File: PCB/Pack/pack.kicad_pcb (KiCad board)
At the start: 2 copper layers, 100 x 100 mm, 45 parts, among them J1 Conn_01x01, J2 Conn_01x01, J3 Conn_01x01, J4 Conn_01x01, J5 Conn_01x01, J6 Conn_01x01, J7 Conn_01x02, J8 Conn_01x02, J9 Conn_01x02

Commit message: Major update 12S10P
3dprintable casing for 12S10P 1.5kWh
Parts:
- removed J4: Conn_01x01, Pin_Headers:Pin_Header_Straight_1x01_Pitch2.54mm
- removed J5, J6: Conn_01x01, ENNOID:Pack
- removed J7, J8, J9: Conn_01x02, Pin_Headers:Pin_Header_Straight_1x02_Pitch2.54mm_SMD_Pin1Left
- added BT1: Battery_Cell, ENNOID:18650, F.Cu at (240.0, 9.12)
- added BT100: Battery_Cell, ENNOID:18650, F.Cu at (180.0, 147.7)
- added BT101: Battery_Cell, ENNOID:18650, F.Cu at (160.0, 147.7)
- added BT102: Battery_Cell, ENNOID:18650, F.Cu at (140.0, 147.7)
- added BT103: Battery_Cell, ENNOID:18650, F.Cu at (120.0, 147.7)
- added BT104: Battery_Cell, ENNOID:18650, F.Cu at (100.0, 147.7)
- added BT105: Battery_Cell, ENNOID:18650, F.Cu at (80.0, 147.7)
- added BT109: Battery_Cell, ENNOID:18650, F.Cu at (230.0, 165.0)
- added BT110: Battery_Cell, ENNOID:18650, F.Cu at (210.0, 165.0)
- added BT111: Battery_Cell, ENNOID:18650, F.Cu at (190.0, 165.0)
- added BT112: Battery_Cell, ENNOID:18650, F.Cu at (170.0, 165.0)
- added BT113: Battery_Cell, ENNOID:18650, F.Cu at (150.0, 165.0)
- added BT114: Battery_Cell, ENNOID:18650, F.Cu at (130.0, 165.0)
- added BT115: Battery_Cell, ENNOID:18650, F.Cu at (110.0, 165.0)
- added BT116: Battery_Cell, ENNOID:18650, F.Cu at (90.0, 165.0)
- added BT117: Battery_Cell, ENNOID:18650, F.Cu at (70.0, 165.0)
- added BT118: Battery_Cell, ENNOID:18650, F.Cu at (50.0, 165.0)
- added BT119: Battery_Cell, ENNOID:18650, F.Cu at (30.0, 165.0)
- added BT120: Battery_Cell, ENNOID:18650, F.Cu at (10.0, 165.0)
- added BT13: Battery_Cell, ENNOID:18650, F.Cu at (230.0, 26.4)
- added BT14: Battery_Cell, ENNOID:18650, F.Cu at (210.0, 26.4)
- added BT15: Battery_Cell, ENNOID:18650, F.Cu at (190.0, 26.4)
- added BT16: Battery_Cell, ENNOID:18650, F.Cu at (170.0, 26.4)
- added BT17: Battery_Cell, ENNOID:18650, F.Cu at (150.0, 26.4)
- added BT18: Battery_Cell, ENNOID:18650, F.Cu at (130.0, 26.4)
- added BT19: Battery_Cell, ENNOID:18650, F.Cu at (110.0, 26.4)
- added BT2: Battery_Cell, ENNOID:18650, F.Cu at (220.0, 9.12)
- added BT20: Battery_Cell, ENNOID:18650, F.Cu at (90.0, 26.4)
- added BT21: Battery_Cell, ENNOID:18650, F.Cu at (70.0, 26.4)
- added BT25: Battery_Cell, ENNOID:18650, F.Cu at (240.0, 43.8)
- added BT26: Battery_Cell, ENNOID:18650, F.Cu at (220.0, 43.8)
- added BT27: Battery_Cell, ENNOID:18650, F.Cu at (200.0, 43.8)
- added BT3: Battery_Cell, ENNOID:18650, F.Cu at (200.0, 9.12)
- added BT37: Battery_Cell, ENNOID:18650, F.Cu at (230.0, 61.1)
- added BT38: Battery_Cell, ENNOID:18650, F.Cu at (210.0, 61.1)
- added BT39: Battery_Cell, ENNOID:18650, F.Cu at (190.0, 61.1)
- added BT4: Battery_Cell, ENNOID:18650, F.Cu at (180.0, 9.12)
- added BT40: Battery_Cell, ENNOID:18650, F.Cu at (170.0, 61.1)
- added BT41: Battery_Cell, ENNOID:18650, F.Cu at (150.0, 61.1)
- added BT42: Battery_Cell, ENNOID:18650, F.Cu at (130.0, 61.1)
- added BT43: Battery_Cell, ENNOID:18650, F.Cu at (110.0, 61.1)
- added BT44: Battery_Cell, ENNOID:18650, F.Cu at (90.0, 61.1)
- added BT45: Battery_Cell, ENNOID:18650, F.Cu at (70.0, 61.1)
- added BT49: Battery_Cell, ENNOID:18650, F.Cu at (240.0, 78.4)
- added BT5: Battery_Cell, ENNOID:18650, F.Cu at (160.0, 9.12)
- added BT50: Battery_Cell, ENNOID:18650, F.Cu at (220.0, 78.4)
- added BT51: Battery_Cell, ENNOID:18650, F.Cu at (200.0, 78.4)
- added BT52: Battery_Cell, ENNOID:18650, F.Cu at (180.0, 78.4)
- added BT53: Battery_Cell, ENNOID:18650, F.Cu at (160.0, 78.4)
- added BT54: Battery_Cell, ENNOID:18650, F.Cu at (140.0, 78.4)
- added BT55: Battery_Cell, ENNOID:18650, F.Cu at (120.0, 78.4)
- added BT56: Battery_Cell, ENNOID:18650, F.Cu at (100.0, 78.4)
- added BT57: Battery_Cell, ENNOID:18650, F.Cu at (80.0, 78.4)
- added BT6: Battery_Cell, ENNOID:18650, F.Cu at (140.0, 9.12)
- added BT61: Battery_Cell, ENNOID:18650, F.Cu at (230.0, 95.7)
- added BT62: Battery_Cell, ENNOID:18650, F.Cu at (210.0, 95.7)
- added BT63: Battery_Cell, ENNOID:18650, F.Cu at (190.0, 95.7)
- added BT64: Battery_Cell, ENNOID:18650, F.Cu at (170.0, 95.7)
- added BT65: Battery_Cell, ENNOID:18650, F.Cu at (150.0, 95.7)
- added BT66: Battery_Cell, ENNOID:18650, F.Cu at (130.0, 95.7)
- added BT67: Battery_Cell, ENNOID:18650, F.Cu at (110.0, 95.7)
- added BT68: Battery_Cell, ENNOID:18650, F.Cu at (90.0, 95.7)
- added BT69: Battery_Cell, ENNOID:18650, F.Cu at (70.0, 95.7)
- added BT7: Battery_Cell, ENNOID:18650, F.Cu at (120.0, 9.12)
- added BT73: Battery_Cell, ENNOID:18650, F.Cu at (240.0, 113.0)
- added BT74: Battery_Cell, ENNOID:18650, F.Cu at (220.0, 113.0)
- added BT75: Battery_Cell, ENNOID:18650, F.Cu at (200.0, 113.0)
- added BT76: Battery_Cell, ENNOID:18650, F.Cu at (180.0, 113.0)
- added BT77: Battery_Cell, ENNOID:18650, F.Cu at (160.0, 113.0)
- added BT78: Battery_Cell, ENNOID:18650, F.Cu at (140.0, 113.0)
- added BT79: Battery_Cell, ENNOID:18650, F.Cu at (120.0, 113.0)
- added BT8: Battery_Cell, ENNOID:18650, F.Cu at (100.0, 9.12)
- added BT80: Battery_Cell, ENNOID:18650, F.Cu at (100.0, 113.0)
- added BT81: Battery_Cell, ENNOID:18650, F.Cu at (80.0, 113.0)
- added BT85: Battery_Cell, ENNOID:18650, F.Cu at (230.0, 130.4)
- added BT86: Battery_Cell, ENNOID:18650, F.Cu at (210.0, 130.4)
- added BT87: Battery_Cell, ENNOID:18650, F.Cu at (190.0, 130.4)
- added BT88: Battery_Cell, ENNOID:18650, F.Cu at (170.0, 130.4)
- added BT89: Battery_Cell, ENNOID:18650, F.Cu at (150.0, 130.4)
- added BT9: Battery_Cell, ENNOID:18650, F.Cu at (80.0, 9.12)
- added BT90: Battery_Cell, ENNOID:18650, F.Cu at (130.0, 130.4)
- added BT91: Battery_Cell, ENNOID:18650, F.Cu at (110.0, 130.4)
- added BT92: Battery_Cell, ENNOID:18650, F.Cu at (90.0, 130.4)
- added BT93: Battery_Cell, ENNOID:18650, F.Cu at (70.0, 130.4)
- added BT97: Battery_Cell, ENNOID:18650, F.Cu at (240.0, 147.7)
- added BT98: Battery_Cell, ENNOID:18650, F.Cu at (220.0, 147.7)
- added BT99: Battery_Cell, ENNOID:18650, F.Cu at (200.0, 147.7)
- added J14: Conn_01x01, ENNOID:Pack, F.Cu at (250.0, 87.0)
- added J15: Conn_01x01, ENNOID:Pack, F.Cu at (0.00, 87.0)
- added LOGO1: Logo_Open_Hardware_Small, ENNOID:ENNOID-LOGO, B.Cu at (126.9, 87.2)
- added TH4: Thermistor, Resistors_SMD:R_0805_HandSoldering, F.Cu at (167.5, 70.4)
- added TH5: Thermistor, Resistors_SMD:R_0805_HandSoldering, F.Cu at (207.4, 35.0)
- BT10: renamed from BT1; moved to F.Cu
- BT106: renamed from BT25; moved to F.Cu
- BT107: renamed from BT26; moved to F.Cu
- BT108: renamed from BT27; moved to F.Cu
- BT11: renamed from BT2; moved to F.Cu
- BT12: renamed from BT3; moved to F.Cu
- BT22: renamed from BT4; moved to F.Cu
- BT23: renamed from BT5; moved to F.Cu
- BT24: renamed from BT6; moved to F.Cu
- BT28, BT29, BT30, BT31, BT32, BT33: footprint ENNOID:half -> ENNOID:18650; moved to F.Cu
- BT34: renamed from BT7; moved to F.Cu
- BT35: renamed from BT8; moved to F.Cu
- BT36: renamed from BT9; moved to F.Cu
- BT46: renamed from BT10; moved to F.Cu
- BT47: renamed from BT11; moved to F.Cu
- BT48: renamed from BT12; moved to F.Cu
- BT58: renamed from BT13; moved to F.Cu
- BT59: renamed from BT14; moved to F.Cu
- BT60: renamed from BT15; moved to F.Cu
- BT70: renamed from BT16; moved to F.Cu
- BT71: renamed from BT17; moved to F.Cu
- BT72: renamed from BT18; moved to F.Cu
- BT82: renamed from BT19; moved to F.Cu
- BT83: renamed from BT20; moved to F.Cu
- BT84: renamed from BT21; moved to F.Cu
- BT94: renamed from BT22; moved to F.Cu
- BT95: renamed from BT23; moved to F.Cu
- BT96: renamed from BT24; moved to F.Cu
- J1, J3: value Conn_01x01 -> Conn_01x13; footprint Pin_Headers:Pin_Header_Straight_1x01_Pitch2.54mm -> Pin_Headers:Pin_Header_Straight_1x13_Pitch2.54mm; moved to F.Cu
- J2: value Conn_01x01 -> Conn_01x10; footprint Pin_Headers:Pin_Header_Straight_1x01_Pitch2.54mm -> Pin_Headers:Pin_Header_Straight_1x10_Pitch2.54mm; moved to F.Cu
- TH1, TH2, TH3: moved to F.Cu
- moved J1 202.0 mm to (127.0, 188.0), turned to 90 degrees
- moved J2 162.0 mm to (98.0, 188.0), turned to 90 degrees
- moved J3 128.6 mm to (157.5, -4.00), turned to 270 degrees
- moved BT106 127.1 mm to (60.0, 147.7), turned to 270 degrees
- moved BT31 124.9 mm to (120.0, 43.8), turned to 270 degrees
- moved BT94 124.8 mm to (50.0, 130.4), turned to 270 degrees
- moved BT107 103.1 mm to (40.0, 147.7), turned to 270 degrees
- moved BT95 101.1 mm to (30.0, 130.4), turned to 270 degrees
- moved BT32 100.0 mm to (100.0, 43.8), turned to 270 degrees
- moved TH2 96.9 mm to (66.6, 105.4)
- moved BT108 90.2 mm to (20.0, 147.7), turned to 270 degrees
- moved BT82 89.5 mm to (60.0, 113.0), turned to 270 degrees
- moved BT96 88.7 mm to (10.0, 130.4)
- moved BT28 87.2 mm to (180.0, 43.8), turned to 270 degrees
- moved BT70 87.1 mm to (50.0, 95.7), turned to 270 degrees
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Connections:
- BT10 pad 1: Net-(BT1-Pad1) -> Net-(BT10-Pad1)
- BT10 pad 2: Net-(BT1-Pad2) -> Net-(BT10-Pad2)
- BT106 pad 1: Net-(BT1-Pad1) -> Net-(BT10-Pad1)
- BT106 pad 2: Net-(BT1-Pad2) -> Net-(BT10-Pad2)
- BT107 pad 1: Net-(BT1-Pad2) -> Net-(BT10-Pad2)
- BT107 pad 2: Net-(BT11-Pad2) -> Net-(BT107-Pad2)
- BT108 pad 1: Net-(BT11-Pad2) -> Net-(BT107-Pad2)
- BT108 pad 2: Net-(BT12-Pad2) -> Net-(BT108-Pad2)
- BT11 pad 1: Net-(BT1-Pad2) -> Net-(BT10-Pad2)
- BT11 pad 2: Net-(BT11-Pad2) -> Net-(BT107-Pad2)
- BT12 pad 1: Net-(BT11-Pad2) -> Net-(BT107-Pad2)
- BT12 pad 2: Net-(BT12-Pad2) -> Net-(BT108-Pad2)
- BT22 pad 1: Net-(BT1-Pad1) -> Net-(BT10-Pad1)
- BT22 pad 2: Net-(BT1-Pad2) -> Net-(BT10-Pad2)
- BT23 pad 1: Net-(BT1-Pad2) -> Net-(BT10-Pad2)
- BT23 pad 2: Net-(BT11-Pad2) -> Net-(BT107-Pad2)
- BT24 pad 1: Net-(BT11-Pad2) -> Net-(BT107-Pad2)
- BT24 pad 2: Net-(BT12-Pad2) -> Net-(BT108-Pad2)
- BT28 pad 1: Net-(BT1-Pad1) -> Net-(BT100-Pad1)
- BT28 pad 2: Net-(BT1-Pad2) -> Net-(BT100-Pad2)
- BT29 pad 1: Net-(BT1-Pad2) -> Net-(BT100-Pad2)
- BT29 pad 2: Net-(BT11-Pad2) -> Net-(BT101-Pad2)
- BT30 pad 1: Net-(BT11-Pad2) -> Net-(BT101-Pad2)
- BT30 pad 2: Net-(BT12-Pad2) -> Net-(BT102-Pad2)
- BT31 pad 1: Net-(BT1-Pad1) -> Net-(BT102-Pad2)
- BT31 pad 2: Net-(BT1-Pad2) -> Net-(BT103-Pad2)
- BT32 pad 1: Net-(BT1-Pad2) -> Net-(BT103-Pad2)
- BT32 pad 2: Net-(BT11-Pad2) -> Net-(BT104-Pad2)
- BT33 pad 1: Net-(BT11-Pad2) -> Net-(BT104-Pad2)
- BT33 pad 2: Net-(BT12-Pad2) -> Net-(BT10-Pad1)
- BT34 pad 1: Net-(BT1-Pad1) -> Net-(BT10-Pad1)
- BT34 pad 2: Net-(BT1-Pad2) -> Net-(BT10-Pad2)
- BT35 pad 1: Net-(BT1-Pad2) -> Net-(BT10-Pad2)
- BT35 pad 2: Net-(BT11-Pad2) -> Net-(BT107-Pad2)
- BT36 pad 1: Net-(BT11-Pad2) -> Net-(BT107-Pad2)
- BT36 pad 2: Net-(BT12-Pad2) -> Net-(BT108-Pad2)
- BT46 pad 1: Net-(BT1-Pad1) -> Net-(BT10-Pad1)
- BT46 pad 2: Net-(BT1-Pad2) -> Net-(BT10-Pad2)
- BT47 pad 1: Net-(BT1-Pad2) -> Net-(BT10-Pad2)
- BT47 pad 2: Net-(BT11-Pad2) -> Net-(BT107-Pad2)
- BT48 pad 1: Net-(BT11-Pad2) -> Net-(BT107-Pad2)
- BT48 pad 2: Net-(BT12-Pad2) -> Net-(BT108-Pad2)
- BT58 pad 1: Net-(BT1-Pad1) -> Net-(BT10-Pad1)
- BT58 pad 2: Net-(BT1-Pad2) -> Net-(BT10-Pad2)
- BT59 pad 1: Net-(BT1-Pad2) -> Net-(BT10-Pad2)
- BT59 pad 2: Net-(BT11-Pad2) -> Net-(BT107-Pad2)
- BT60 pad 1: Net-(BT11-Pad2) -> Net-(BT107-Pad2)
- BT60 pad 2: Net-(BT12-Pad2) -> Net-(BT108-Pad2)
- BT70 pad 1: Net-(BT1-Pad1) -> Net-(BT10-Pad1)
- BT70 pad 2: Net-(BT1-Pad2) -> Net-(BT10-Pad2)
- BT71 pad 1: Net-(BT1-Pad2) -> Net-(BT10-Pad2)
- BT71 pad 2: Net-(BT11-Pad2) -> Net-(BT107-Pad2)
- BT72 pad 1: Net-(BT11-Pad2) -> Net-(BT107-Pad2)
- BT72 pad 2: Net-(BT12-Pad2) -> Net-(BT108-Pad2)
- BT82 pad 1: Net-(BT1-Pad1) -> Net-(BT10-Pad1)
- BT82 pad 2: Net-(BT1-Pad2) -> Net-(BT10-Pad2)
- BT83 pad 1: Net-(BT1-Pad2) -> Net-(BT10-Pad2)
- BT83 pad 2: Net-(BT11-Pad2) -> Net-(BT107-Pad2)
- BT84 pad 1: Net-(BT11-Pad2) -> Net-(BT107-Pad2)
- BT84 pad 2: Net-(BT12-Pad2) -> Net-(BT108-Pad2)
- BT94 pad 1: Net-(BT1-Pad1) -> Net-(BT10-Pad1)
- BT94 pad 2: Net-(BT1-Pad2) -> Net-(BT10-Pad2)
- BT95 pad 1: Net-(BT1-Pad2) -> Net-(BT10-Pad2)
- BT95 pad 2: Net-(BT11-Pad2) -> Net-(BT107-Pad2)
- BT96 pad 1: Net-(BT11-Pad2) -> Net-(BT107-Pad2)
- BT96 pad 2: Net-(BT12-Pad2) -> Net-(BT108-Pad2)
- J1 pad 1: Net-(BT1-Pad1) -> Net-(BT108-Pad2)
- J2 pad 1: Net-(BT1-Pad2) -> Net-(J2-Pad1)
- J3 pad 1: Net-(BT11-Pad2) -> Net-(BT1-Pad1)
- TH1 pad 1: Net-(J7-Pad1) -> Net-(J2-Pad1)
- TH1 pad 2: Net-(J7-Pad2) -> Net-(J2-Pad2)
- TH2 pad 1: Net-(J9-Pad1) -> Net-(J2-Pad3)
- TH2 pad 2: Net-(J9-Pad2) -> Net-(J2-Pad4)
- TH3 pad 1: Net-(J8-Pad1) -> Net-(J2-Pad5)
- TH3 pad 2: Net-(J8-Pad2) -> Net-(J2-Pad6)
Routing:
- net Net-(BT108-Pad2): track 0.00 -> 488.5 mm
- net Net-(BT107-Pad2): track 0.00 -> 467.9 mm
- net Net-(BT10-Pad2): track 0.00 -> 433.5 mm
- net Net-(BT10-Pad1): track 0.00 -> 393.3 mm
- net Net-(BT1-Pad2): track 0.00 -> 383.7 mm, vias 200 -> 0
- net Net-(BT1-Pad1): track 0.00 -> 372.0 mm
- net Net-(BT110-Pad2): track 0.00 -> 360.3 mm
- net Net-(BT104-Pad2): track 0.00 -> 359.3 mm
- net Net-(BT103-Pad2): track 0.00 -> 318.0 mm
- net Net-(BT100-Pad1): track 0.00 -> 308.5 mm
- net Net-(BT102-Pad2): track 0.00 -> 304.4 mm
- net Net-(BT100-Pad2): track 0.00 -> 295.0 mm
- net Net-(BT101-Pad2): track 0.00 -> 285.8 mm
- net Net-(J2-Pad9): track 0.00 -> 212.6 mm, vias 0 -> 1
- net Net-(J2-Pad10): track 0.00 -> 209.3 mm, vias 0 -> 1
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- removed copper zone on B.Cu, net Net-(BT1-Pad1)
- removed copper zone on B.Cu, net Net-(BT1-Pad2)
- removed copper zone on F.Cu, net Net-(BT1-Pad2)
- removed copper zone on B.Cu, net Net-(BT11-Pad2)
- removed copper zone on F.Cu, net Net-(BT11-Pad2)
- removed copper zone on F.Cu, net Net-(BT12-Pad2)
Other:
- board size 100 x 100 mm -> 250 x 199 mm
- board text removed: "C0 C3 C6 C9 C12 C15"
- board text removed: "C1 C4 C7 C10 C13 C16"
- board text removed: "C12"
- board text removed: "C18"
- board text removed: "C2 C5 C8 C11 C14 C17"
- board text removed: "ENNOID"
- board text removed: "https://github.com/EnnoidMe/ENNOID-PACK"

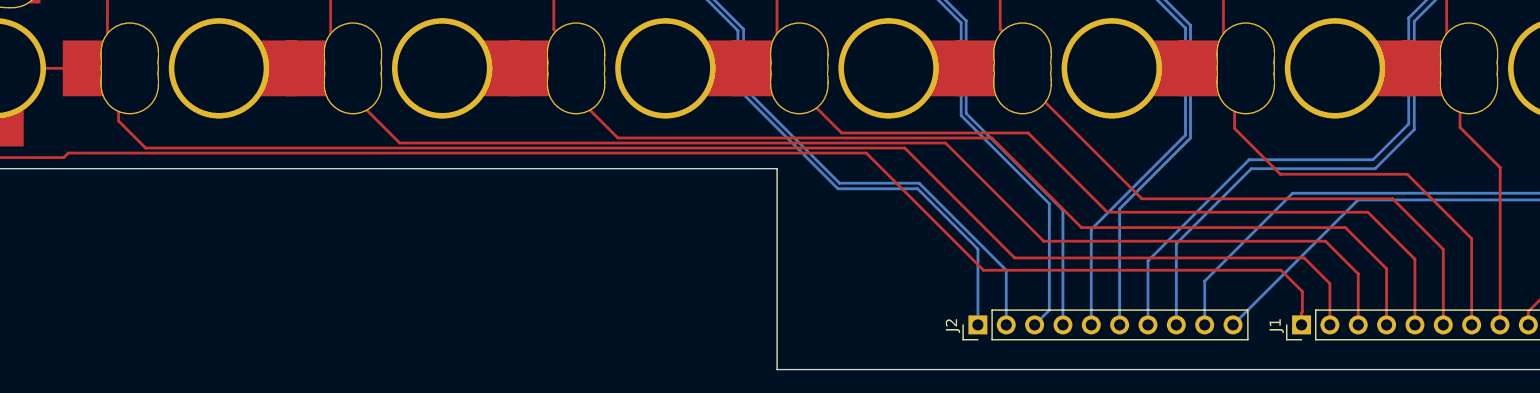
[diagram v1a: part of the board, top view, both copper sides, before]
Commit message: small changes to top pcb
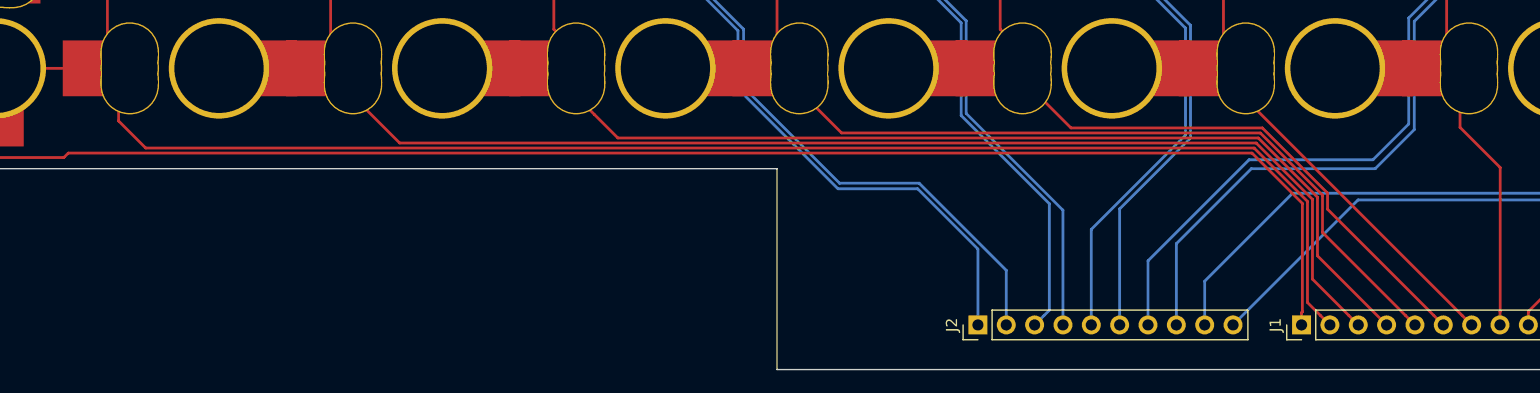
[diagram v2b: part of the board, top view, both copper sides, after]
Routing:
- net Net-(BT102-Pad2): track 304.4 -> 297.7 mm
- net Net-(BT108-Pad2): track 488.5 -> 493.2 mm
- net Net-(BT107-Pad2): track 467.9 -> 471.0 mm
- net Net-(BT103-Pad2): track 318.0 -> 314.9 mm
- net Net-(BT10-Pad2): track 433.5 -> 435.0 mm
- net Net-(BT104-Pad2): track 359.3 -> 357.8 mm
